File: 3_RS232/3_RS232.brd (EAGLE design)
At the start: 67.4 x 44.8 mm, 8 parts, among them IC5 MAX211ECWI, X9 ALLSERIALD

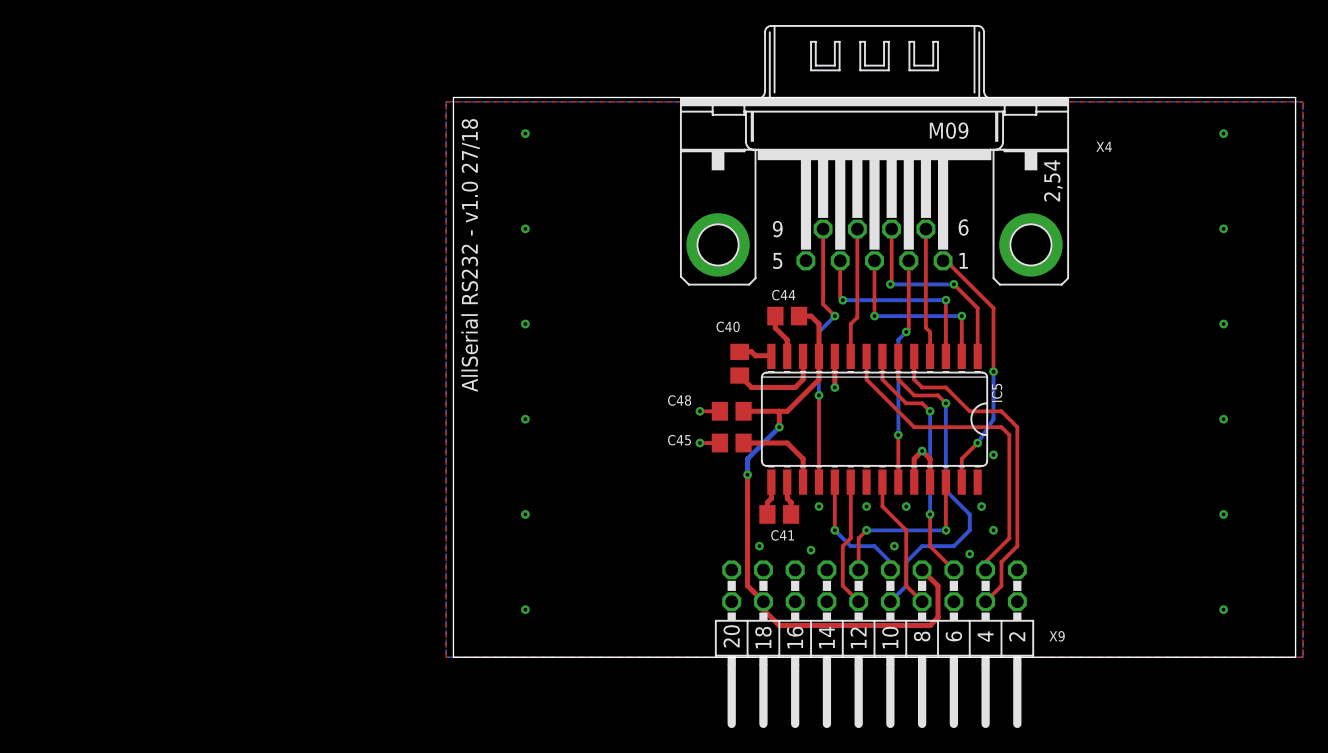
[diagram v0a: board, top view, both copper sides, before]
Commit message: final design & order
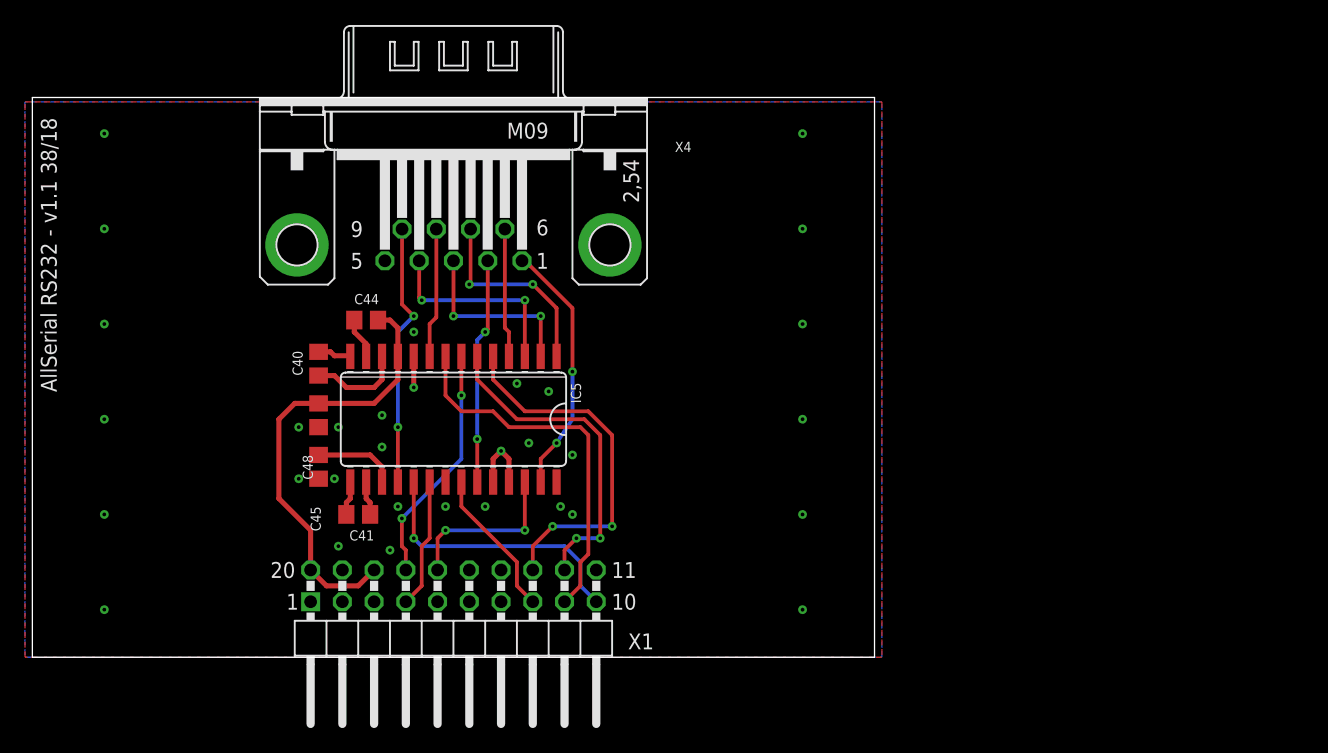
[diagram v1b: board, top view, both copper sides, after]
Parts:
- removed X9: ALLSERIALD, AllSerial:DAUGHTER-THT
- added X1: ALLSERIALSLAVE, AllSerialv2:DAUGHTER-THT
- moved C44 33.7 mm to (-6.99, 27.0)
- moved C40 33.7 mm to (-10.8, 23.5)
- moved IC5 33.7 mm to (0.00, 19.1)
- moved X4 33.7 mm to (0.00, 33.0)
- moved C41 33.7 mm to (-7.62, 11.4)
- moved C45 33.1 mm to (-10.8, 15.2), turned to 270 degrees
- moved C48 33.1 mm to (-10.8, 19.4), turned to 270 degrees
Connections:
- net +5V: now also X1.18, X1.20; no longer X9.18, X9.7
- net GND: now also X1.1; no longer X9.19
- net N$100: now also X1.12; no longer X9.10
- net N$93: now also X1.17; no longer X9.5
- net N$94: now also X1.8; no longer X9.8
- net N$95: now also X1.4; no longer X9.12
- net N$96: now also X1.9; no longer X9.3
- net N$97: now also X1.16; no longer X9.11
- net N$98: now also X1.10; no longer X9.9
- net N$99: now also X1.13; no longer X9.4
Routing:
- net +5V: track 49.9 -> 36.1 mm, vias 2 -> 0
- net N$98: track 9.99 -> 22.3 mm
- net N$96: track 26.7 -> 30.0 mm
- net GND: track 11.2 -> 7.99 mm, vias 26 -> 32
- net N$99: track 26.7 -> 29.4 mm, vias 0 -> 2
- net N$94: track 10.9 -> 11.9 mm
- net N$93: track 20.2 -> 19.2 mm
- net N$100: track 27.2 -> 26.6 mm, vias 1 -> 2
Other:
- board text added: "AllSerial RS232 - v1.1 38/18"
- board text removed: "AllSerial RS232 - v1.0 27/18"
